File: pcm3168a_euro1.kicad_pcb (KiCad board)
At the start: 2 copper layers, 160 parts, among them J1 Conn_02x04_Odd_Even, J10 Conn_Coaxial, J11 Conn_Coaxial, J12 Conn_Coaxial, J13 Conn_Coaxial, J14 Conn_Coaxial, J15 Conn_Coaxial, J16 Conn_Coaxial, J17 Conn_02x08_Odd_Even, J18 Conn_Coaxial, J2 Conn_02x04_Odd_Even, J3 Conn_02x04_Odd_Even, J4 Conn_02x04_Odd_Even, J5 Conn_02x04_Odd_Even, J6 Conn_Coaxial, J7 Conn_Coaxial, J8 Conn_01x02_Pin, J9 Conn_Coaxial, U1 PCM3168APAPR, U10 74LVC1G17, U11 TLV1117-33, U12 OPA1637, U2 74LVC1G17, U3 74LVC1G17, U4 74LVC1G17, U5 74LVC1G17, U6 74LVC1G17, U7 74LVC1G17, U8 74LVC1G17, U9 74LVC1G17, Y1 SG-210STF 24.5760ML0

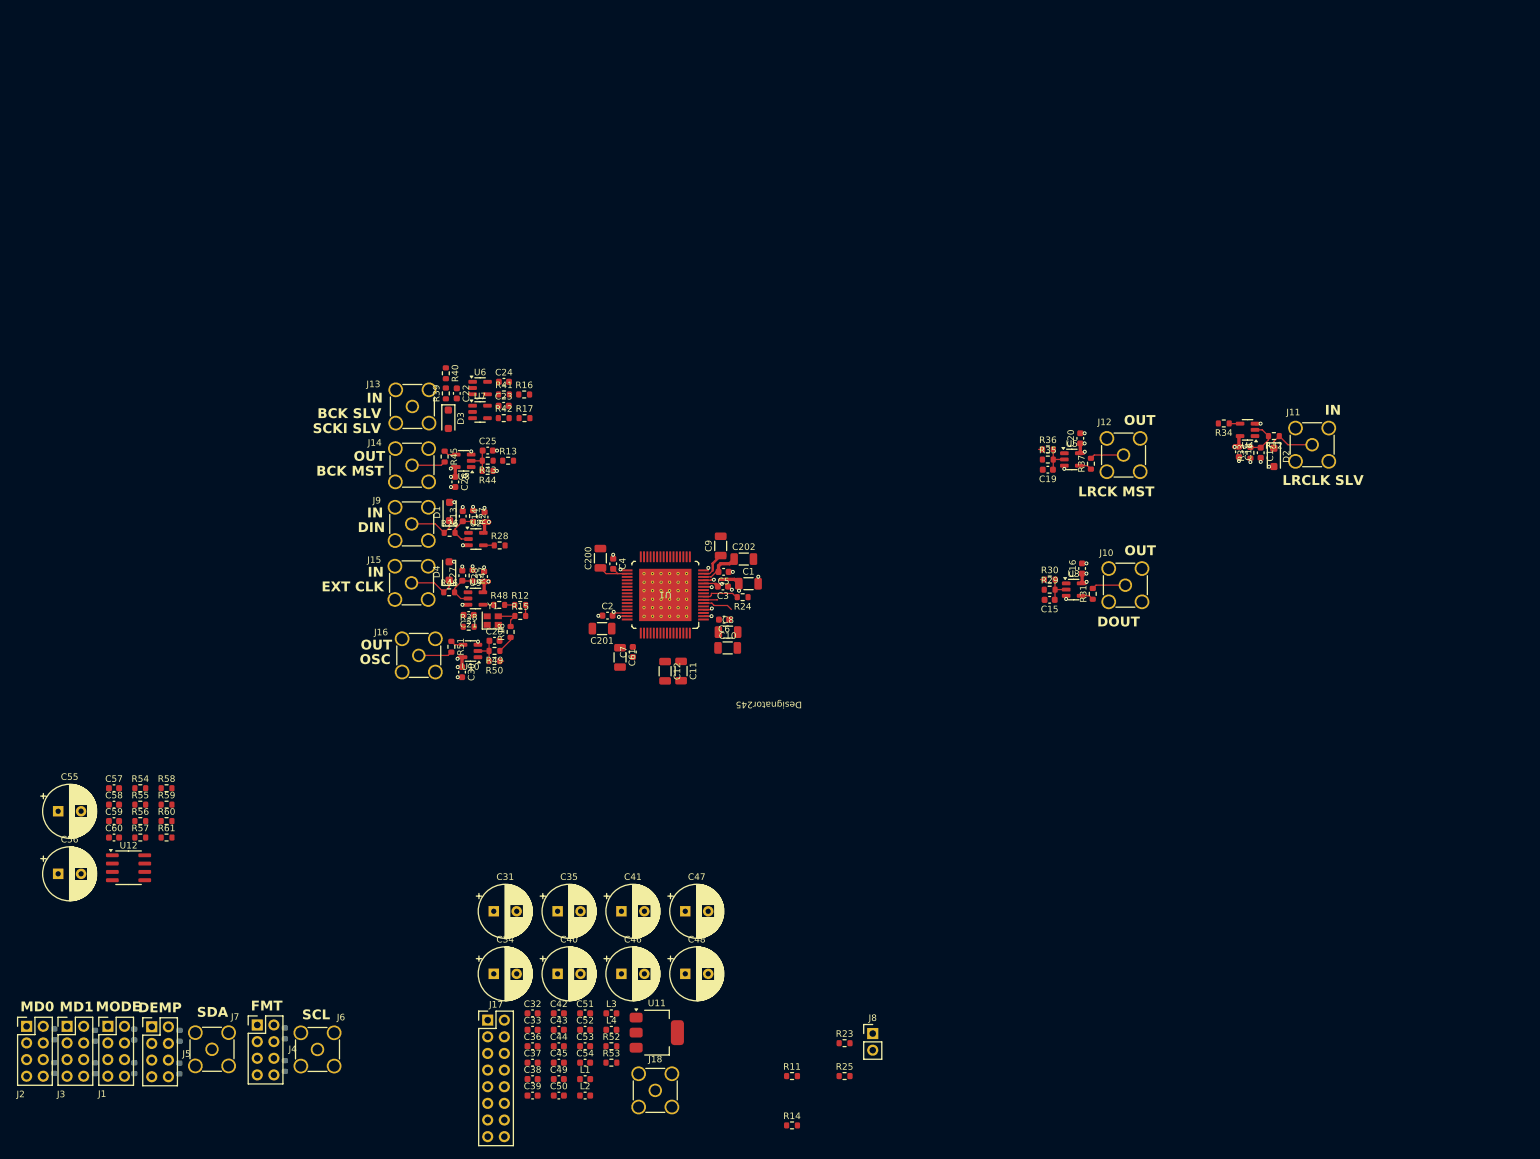
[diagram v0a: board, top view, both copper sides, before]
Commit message: redoing file add
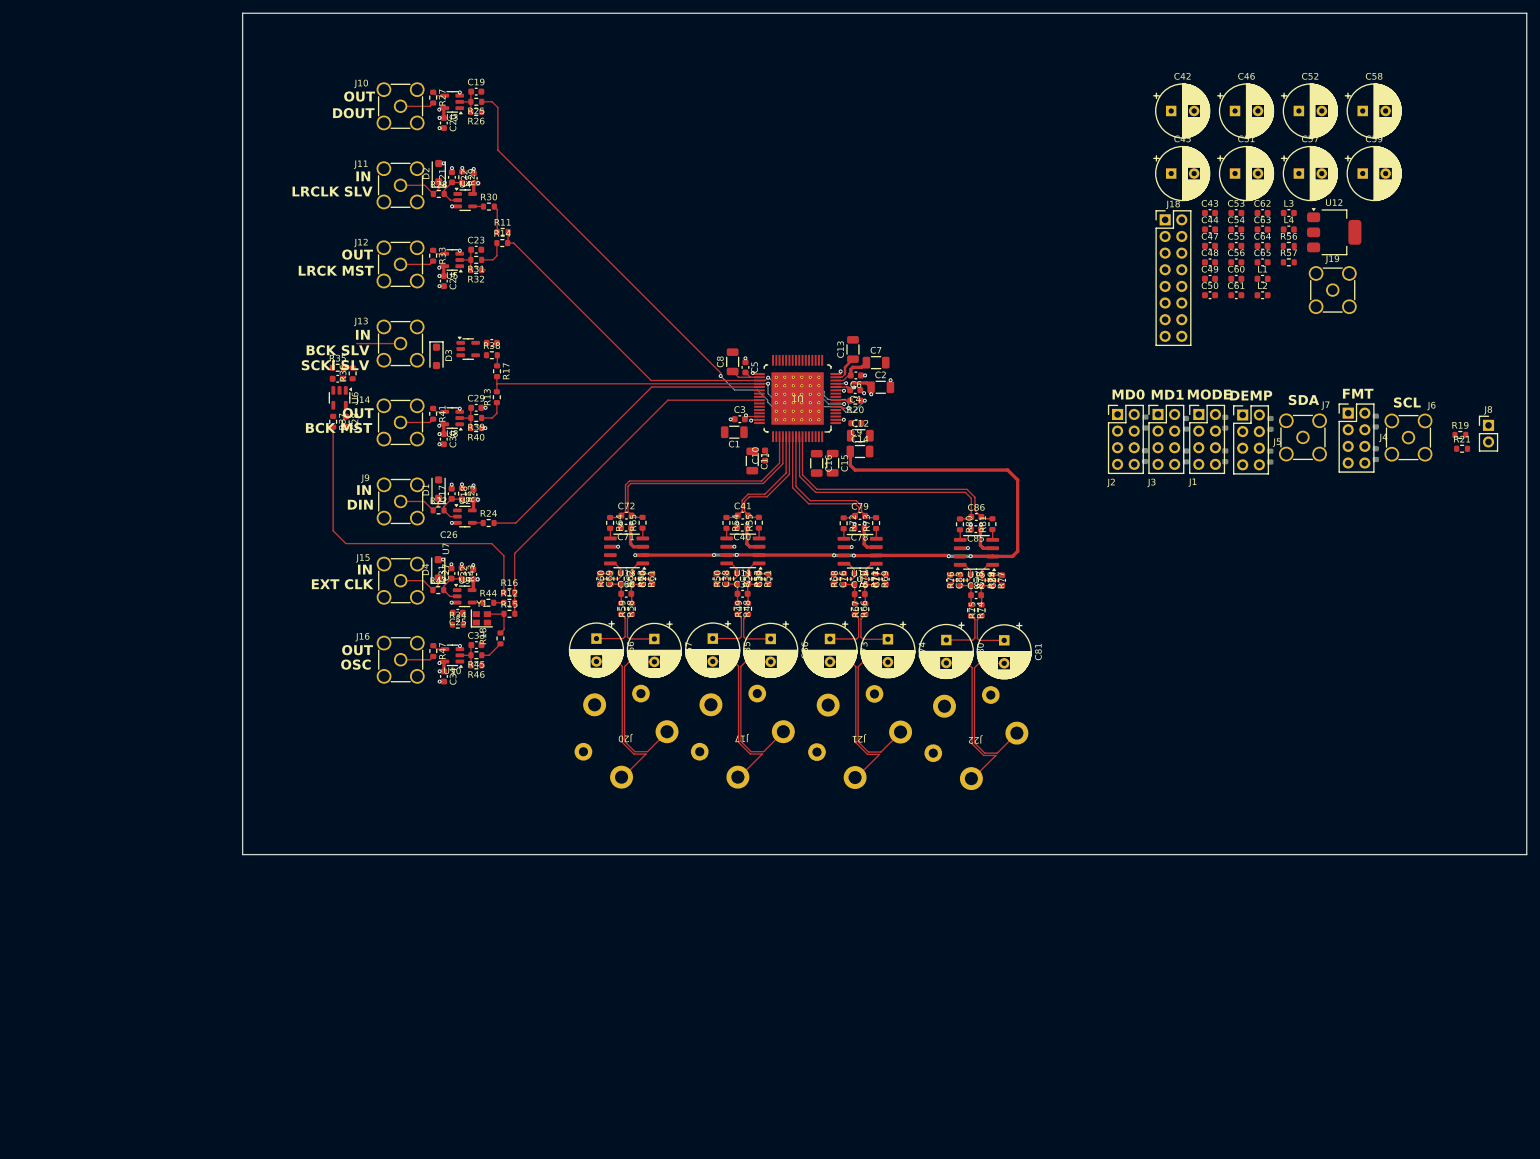
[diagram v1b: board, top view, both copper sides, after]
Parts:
- added C35: C_Polarized_Small, Capacitor_THT:CP_Radial_D8.0mm_P3.50mm, F.Cu at (123.3, 118.6)
- added C36: C_Polarized_Small, Capacitor_THT:CP_Radial_D8.0mm_P3.50mm, F.Cu at (132.1, 118.6)
- added C37: 6.8n, Capacitor_SMD:C_0603_1608Metric, F.Cu at (127.8, 111.7)
- added C38: 1n, Capacitor_SMD:C_0603_1608Metric, F.Cu at (123.8, 109.4)
- added C39: 1n, Capacitor_SMD:C_0603_1608Metric, F.Cu at (131.8, 109.5)
- added C40: 100nF, Capacitor_SMD:C_0603_1608Metric, F.Cu at (127.8, 101.6)
- added C41: 39n, Capacitor_SMD:C_0603_1608Metric, F.Cu at (127.9, 99.8)
- added C71: 100nF, Capacitor_SMD:C_0603_1608Metric, F.Cu at (110.0, 101.6)
- added C73: C_Polarized_Small, Capacitor_THT:CP_Radial_D8.0mm_P3.50mm, F.Cu at (141.2, 118.6)
- added C74: C_Polarized_Small, Capacitor_THT:CP_Radial_D8.0mm_P3.50mm, F.Cu at (150.0, 118.7)
- added C75: 6.8n, Capacitor_SMD:C_0603_1608Metric, F.Cu at (145.7, 111.8)
- added C76: 1n, Capacitor_SMD:C_0603_1608Metric, F.Cu at (141.7, 109.5)
- added C77: 1n, Capacitor_SMD:C_0603_1608Metric, F.Cu at (149.7, 109.5)
- added C78: 100nF, Capacitor_SMD:C_0603_1608Metric, F.Cu at (145.7, 101.7)
- added C79: 39n, Capacitor_SMD:C_0603_1608Metric, F.Cu at (145.8, 99.8)
- added C80: C_Polarized_Small, Capacitor_THT:CP_Radial_D8.0mm_P3.50mm, F.Cu at (158.9, 118.8)
- added C81: C_Polarized_Small, Capacitor_THT:CP_Radial_D8.0mm_P3.50mm, F.Cu at (167.8, 118.8)
- added C82: 6.8n, Capacitor_SMD:C_0603_1608Metric, F.Cu at (163.5, 111.9)
- added C83: 1n, Capacitor_SMD:C_0603_1608Metric, F.Cu at (159.5, 109.7)
- added C84: 1n, Capacitor_SMD:C_0603_1608Metric, F.Cu at (167.4, 109.7)
- added C85: 100nF, Capacitor_SMD:C_0603_1608Metric, F.Cu at (163.4, 101.9)
- added C86: 39n, Capacitor_SMD:C_0603_1608Metric, F.Cu at (163.5, 100.0)
- added J17: ACJS-MV35-3, pcm3168a_euro1:Amphenol_ACJS, F.Cu at (127.7, 133.3)
- added J20: ACJS-MV35-3, pcm3168a_euro1:Amphenol_ACJS, F.Cu at (109.9, 133.3)
- added J21: ACJS-MV35-3, pcm3168a_euro1:Amphenol_ACJS, F.Cu at (145.6, 133.4)
- added J22: ACJS-MV35-3, pcm3168a_euro1:Amphenol_ACJS, F.Cu at (163.3, 133.6)
- added R48: 1.1k, Resistor_SMD:R_0603_1608Metric, F.Cu at (127.1, 114.0)
- added R49: 1.1k, Resistor_SMD:R_0603_1608Metric, F.Cu at (128.7, 114.0)
- added R50: 1.1k, Resistor_SMD:R_0603_1608Metric, F.Cu at (125.4, 109.4)
- added R51: 1.1k, Resistor_SMD:R_0603_1608Metric, F.Cu at (130.2, 109.5)
- added R52: 560, Resistor_SMD:R_0603_1608Metric, F.Cu at (127.0, 109.4)
- added R53: 560, Resistor_SMD:R_0603_1608Metric, F.Cu at (128.7, 109.4)
- added R54: 47, Resistor_SMD:R_0603_1608Metric, F.Cu at (125.4, 100.9)
- added R55: 47, Resistor_SMD:R_0603_1608Metric, F.Cu at (130.3, 100.9)
- added R66: 1.1k, Resistor_SMD:R_0603_1608Metric, F.Cu at (145.0, 114.1)
- added R67: 1.1k, Resistor_SMD:R_0603_1608Metric, F.Cu at (146.6, 114.1)
- added R68: 1.1k, Resistor_SMD:R_0603_1608Metric, F.Cu at (143.3, 109.5)
- added R69: 1.1k, Resistor_SMD:R_0603_1608Metric, F.Cu at (148.1, 109.5)
- added R70: 560, Resistor_SMD:R_0603_1608Metric, F.Cu at (144.9, 109.5)
- added R71: 560, Resistor_SMD:R_0603_1608Metric, F.Cu at (146.6, 109.5)
- added R72: 47, Resistor_SMD:R_0603_1608Metric, F.Cu at (143.3, 101.0)
- added R73: 47, Resistor_SMD:R_0603_1608Metric, F.Cu at (148.2, 100.9)
- added R74: 1.1k, Resistor_SMD:R_0603_1608Metric, F.Cu at (162.7, 114.2)
- added R75: 1.1k, Resistor_SMD:R_0603_1608Metric, F.Cu at (164.3, 114.2)
- added R76: 1.1k, Resistor_SMD:R_0603_1608Metric, F.Cu at (161.1, 109.6)
- added R77: 1.1k, Resistor_SMD:R_0603_1608Metric, F.Cu at (165.9, 109.7)
- added R78: 560, Resistor_SMD:R_0603_1608Metric, F.Cu at (162.6, 109.6)
- added R79: 560, Resistor_SMD:R_0603_1608Metric, F.Cu at (164.3, 109.7)
- added R80: 47, Resistor_SMD:R_0603_1608Metric, F.Cu at (161.0, 101.1)
- added R81: 47, Resistor_SMD:R_0603_1608Metric, F.Cu at (166.0, 101.1)
- added U11: OPA1637, Package_SO:SOIC-8_3.9x4.9mm_P1.27mm, F.Cu at (127.9, 105.2)
- added U14: OPA1637, Package_SO:SOIC-8_3.9x4.9mm_P1.27mm, F.Cu at (145.8, 105.2)
- added U15: OPA1637, Package_SO:SOIC-8_3.9x4.9mm_P1.27mm, F.Cu at (163.5, 105.4)
- moved J1 190.9 mm to (197.5, 84.4)
- moved J2 190.9 mm to (185.1, 84.4)
- moved J3 190.9 mm to (191.2, 84.4)
- moved J4 190.9 mm to (220.3, 84.1)
- moved J5 190.9 mm to (204.2, 84.4)
- moved J7 190.9 mm to (213.4, 87.9)
- moved R1 190.9 mm to (201.5, 85.6)
- moved R10 190.9 mm to (208.4, 90.8)
- moved R4 190.9 mm to (201.5, 90.7)
- moved R5 190.9 mm to (189.3, 90.7)
- moved R6 190.9 mm to (195.5, 90.8)
- moved R7 190.9 mm to (224.5, 85.4)
- moved R8 190.9 mm to (208.4, 85.8)
- moved R9 190.9 mm to (224.5, 90.4)
- moved J6 190.9 mm to (229.5, 87.9)
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- renumbered C201 to C1, C7 to C10, C61 to C11, C8 to C12, C9 to C13, C10 to C14, C11 to C15, C12 to C16, C13 to C17, C14 to C18, C15 to C19, C1 to C2, C16 to C20, C17 to C21, C18 to C22, C19 to C23, C20 to C24, C21 to C25, C22 to C26, C23 to C27, C24 to C28, C25 to C29, C2 to C3, C26 to C30, C27 to C31, C28 to C32, C29 to C33, C30 to C34, C3 to C4, C31 to C42, C32 to C43, C33 to C44, C34 to C45, C35 to C46, C36 to C47, C37 to C48, C38 to C49, C4 to C5, C39 to C50, C40 to C51, C41 to C52, C42 to C53, C43 to C54, C44 to C55, C45 to C56, C46 to C57, C47 to C58, C48 to C59, C5 to C6, C49 to C60, C50 to C61, C51 to C62, C52 to C63, C53 to C64, C54 to C65, C55 to C66, C56 to C67, C57 to C68, C58 to C69, C202 to C7, C59 to C70, C60 to C72, C200 to C8, C6 to C9, J17 to J18, J18 to J19, R23 to R19, R24 to R20, R25 to R21, R26 to R22, R27 to R23, R28 to R24, R29 to R25, R30 to R26, R31 to R27, R32 to R28, R33 to R29, R34 to R30, R35 to R31, R36 to R32, R37 to R33, R38 to R34, R39 to R35, R40 to R36, R41 to R37, R42 to R38, R43 to R39, R44 to R40, R45 to R41, R46 to R42, R47 to R43, R48 to R44, R49 to R45, R50 to R46, R51 to R47, R52 to R56, R53 to R57, R54 to R58, R55 to R59, R56 to R60, R57 to R61, R58 to R62, R59 to R63, R60 to R64, R61 to R65, U11 to U12, U12 to U13
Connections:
- C14 pad 1: Net-(U1-VCOMAD) -> VCOMAD
- C66 pad 2: unconnected-(C55-Pad2) -> Net-(J20-Pin_4)
- C67 pad 2: unconnected-(C56-Pad2) -> Net-(J20-Pin_3)
- C72 pad 1: Net-(C60-Pad1) -> /VIN1-
- C72 pad 2: Net-(C60-Pad2) -> /VIN1+
- R64 pad 1: Net-(C60-Pad1) -> /VIN1-
- R65 pad 2: Net-(C60-Pad2) -> /VIN1+
- U1 pad 1: Net-(U1-VCOMAD) -> VCOMAD
- U1 pad 51: unconnected-(U1-VIN1--Pad51) -> /VIN1-
- U1 pad 52: unconnected-(U1-VIN1+-Pad52) -> /VIN1+
- U1 pad 53: unconnected-(U1-VIN2--Pad53) -> /VIN2-
- U1 pad 54: unconnected-(U1-VIN2+-Pad54) -> /VIN2+
- U1 pad 55: unconnected-(U1-VIN3--Pad55) -> /VIN3-
- U1 pad 56: unconnected-(U1-VIN3+-Pad56) -> /VIN3+
- U1 pad 57: unconnected-(U1-VIN4--Pad57) -> /VIN4-
- U1 pad 58: unconnected-(U1-VIN4+-Pad58) -> /VIN4+
- U1 pad 61: unconnected-(U1-VIN5--Pad61) -> /VIN5-
- U1 pad 62: unconnected-(U1-VIN5+-Pad62) -> /VIN5+
- U1 pad 63: unconnected-(U1-VIN6--Pad63) -> /VIN6-
- U1 pad 64: unconnected-(U1-VIN6+-Pad64) -> /VIN6+
- U13 pad 2: /amp/VOCM -> VCOMAD
- U13 pad 3: unconnected-(U12-V+-Pad3) -> +5V
- U13 pad 6: unconnected-(U12-V--Pad6) -> GND
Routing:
- net VCOMAD: track 0.00 -> 100.6 mm, vias 0 -> 7
- net /dout1/IN: track 0.00 -> 83.7 mm, vias 0 -> 2
- net /LRCK: track 4.67 -> 67.9 mm, vias 0 -> 2
- net /BCK: track 2.14 -> 58.8 mm, vias 0 -> 2
- net /SCKI: track 1.68 -> 56.3 mm
- net /din1/OUT: track 0.00 -> 49.1 mm
- net /mclk/OUT1: track 0.00 -> 49.0 mm
- net /VIN4+: track 0.00 -> 38.8 mm
- net /VIN4-: track 0.00 -> 38.4 mm
- net /VIN1-: track 0.00 -> 35.7 mm
- net /VIN1+: track 0.00 -> 35.7 mm
- net Net-(J20-Pin_4): track 0.00 -> 25.4 mm
- net Net-(J17-Pin_4): track 0.00 -> 25.4 mm
- net Net-(J22-Pin_4): track 0.00 -> 25.4 mm
- net Net-(J21-Pin_4): track 0.00 -> 25.4 mm
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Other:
- board outline added: 196 x 128.4 mm
